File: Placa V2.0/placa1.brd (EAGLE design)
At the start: 35.2 x 55.9 mm, 7 parts, among them IC1 LD117AS50TR

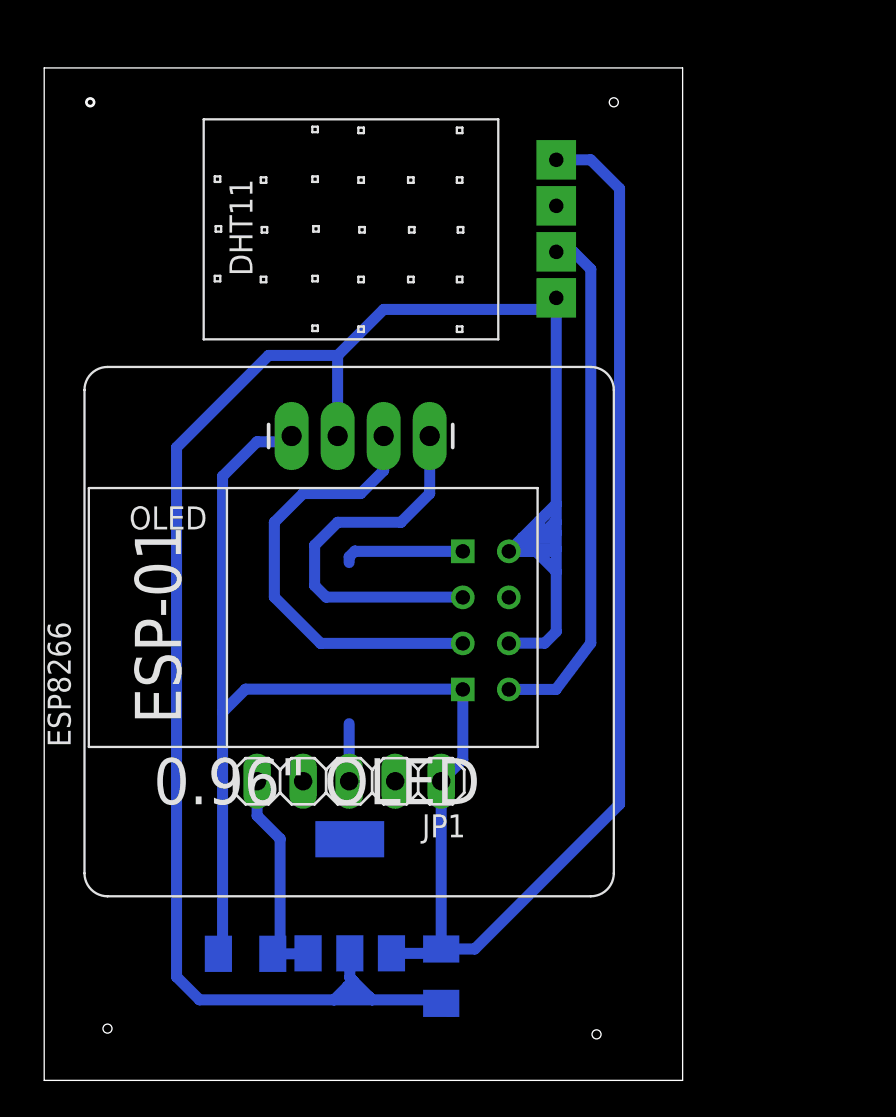
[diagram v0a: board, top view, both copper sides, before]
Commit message: cambios en placa
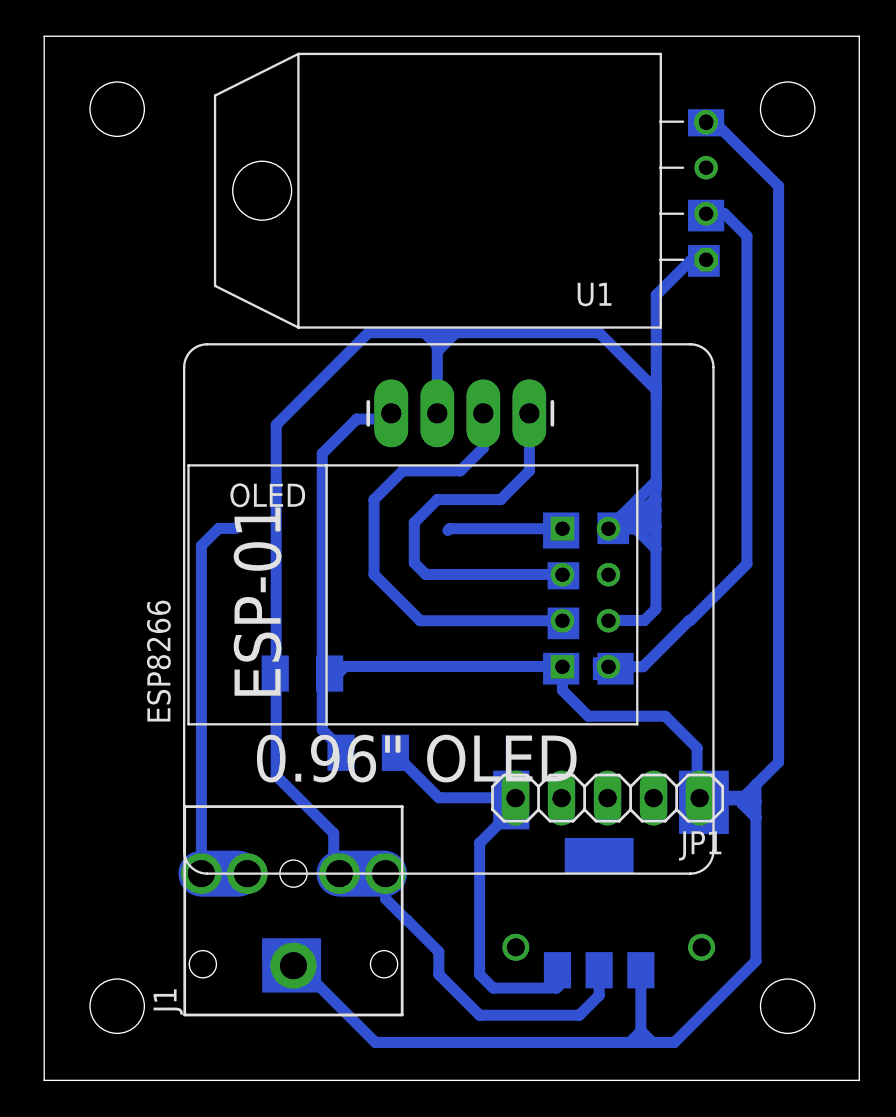
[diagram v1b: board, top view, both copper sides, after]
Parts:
- removed U$1: (no value), DHT11:DHT11
- added J1: STEREOJACKSJ1-352XNG, Ai_Connectors:SJ1-352XNG
- added U1: (no value), dht22:RHT03_DHT-22/RA
- moved C2 18.4 mm to (16.5, 24.4), turned to 180 degrees
- moved JP1 14.3 mm to (33.3, 17.5)
- moved IC1 13.8 mm to (32.8, 11.1)
- moved C1 13.0 mm to (20.1, 20.0)
- moved ESP8266 5.64 mm to (25.2, 28.6)
- moved OLED 5.64 mm to (21.4, 38.7)
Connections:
- removed net N$4: ESP8266.RX, JP1.3
- new net RX: ESP8266.RX, J1.RNG, J1.RSH
- net 3V3: now also J1.TIP, J1.TSH, U1.VDD; no longer U$1.VCC
- net DATA: now also U1.DATA; no longer U$1.DATA
- net GND: now also J1.GND, U1.GND; no longer U$1.GND
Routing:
- net RX: track 0.00 -> 29.3 mm
- net GND: track 113.9 -> 138.8 mm
- net 5V: track 12.2 -> 24.8 mm
- net N$4: track 9.90 -> 0.00 mm, vias 0 -> 1
- net 3V3: track 118.0 -> 125.5 mm
- net DATA: track 28.7 -> 30.8 mm
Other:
- board size 35.2 x 55.9 mm -> 45 x 57.6 mm
